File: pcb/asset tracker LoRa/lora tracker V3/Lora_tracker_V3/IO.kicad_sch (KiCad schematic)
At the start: 14 parts

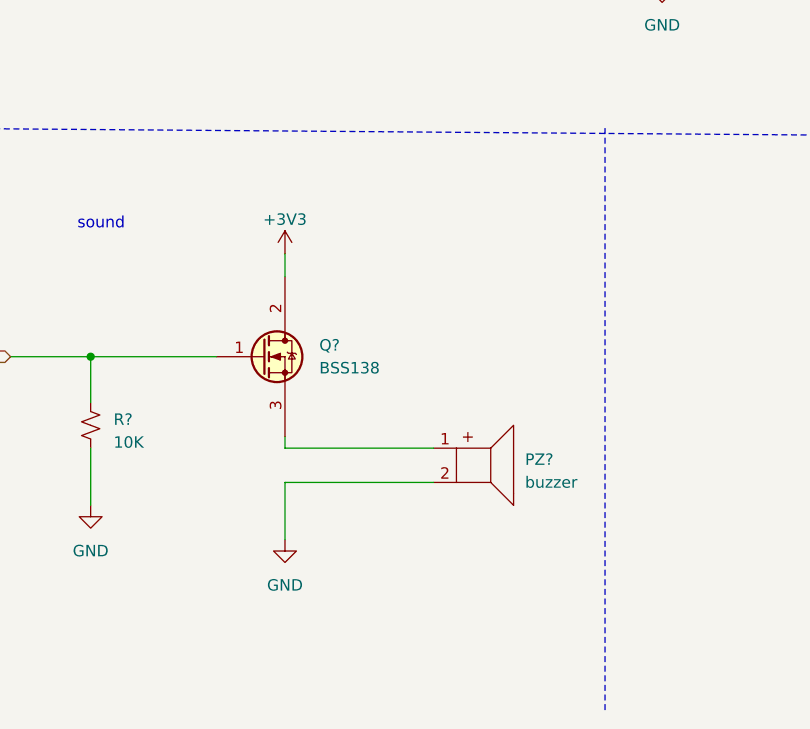
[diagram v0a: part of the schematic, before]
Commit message: sdf
fsgv
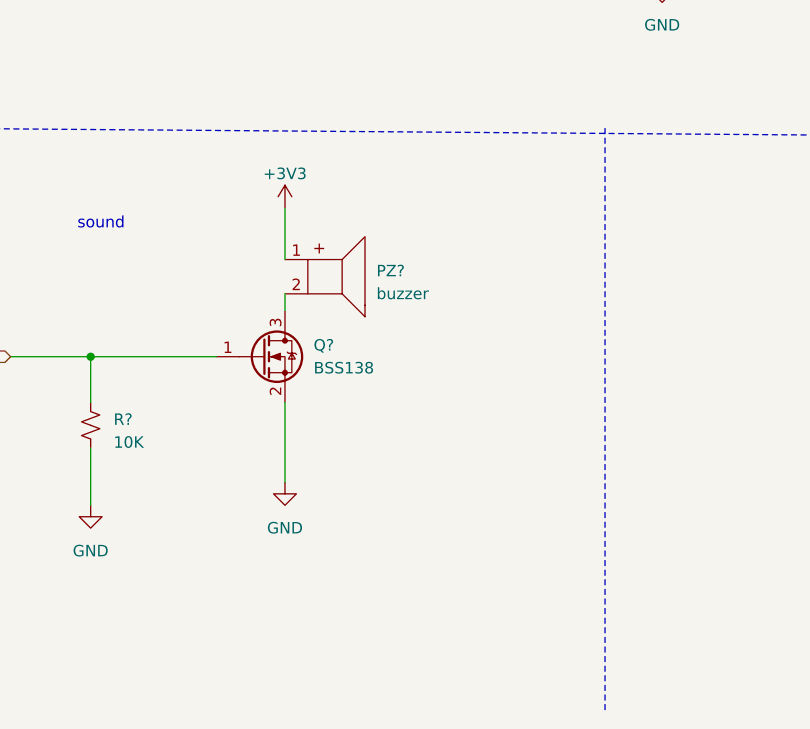
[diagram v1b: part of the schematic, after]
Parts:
- removed Q?: BSS138, halfgeleiders:sot-23,, symbol Halfgelijders:BSS138
- added Q?: BSS138, Package_TO_SOT_SMD:SOT-23, symbol Transistor_FET:BSS138
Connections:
- net +3V3: now also PZ?.1
- net BUZZER: now also Q?.1 (G)
- net GND: now also Q?.2 (S); no longer PZ?.2
- new net: PZ?.2, Q?.3 (D)
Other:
- moved on the sheet: PZ?
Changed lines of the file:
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@@
     (stroke (width 0) (type solid) (color 0 0 0 0))
   )
-  (wire (pts (xy 55.245 148.59) (xy 55.245 151.13))
-    (stroke (width 0) (type solid) (color 0 0 0 0))
-  )
-  (wire (pts (xy 55.245 168.91) (xy 55.245 170.18))
-    (stroke (width 0) (type solid) (color 0 0 0 0))
-  )
-  (wire (pts (xy 55.245 170.18) (xy 71.755 170.18))
-    (stroke (width 0) (type solid) (color 0 0 0 0))
-  )
-  (wire (pts (xy 55.245 173.99) (xy 55.245 180.34))
+  (wire (pts (xy 55.245 143.51) (xy 55.245 149.225))
+    (stroke (width 0) (type solid) (color 0 0 0 0))
+  )
+  (wire (pts (xy 55.245 153.035) (xy 55.245 154.94))
+    (stroke (width 0) (type solid) (color 0 0 0 0))
+  )
+  (wire (pts (xy 55.245 173.99) (xy 55.245 165.1))
     (stroke (width 0) (type solid) (color 0 0 0 0))
   )
@@
   )
   (wire (pts (xy 71.755 80.01) (xy 78.105 80.01))
-    (stroke (width 0) (type solid) (color 0 0 0 0))
-  )
-  (wire (pts (xy 71.755 173.99) (xy 55.245 173.99))
     (stroke (width 0) (type solid) (color 0 0 0 0))
   )
@@
     (effects (font (size 1.27 1.27)) (justify right))
   )
-  (symbol (lib_id "power:+3V3") (at 55.245 148.59 0) (unit 1)
-    (in_bom yes) (on_board yes)
-    (property "Reference" "#PWR?" (id 0) (at 55.245 152.4 0)
-      (effects (font (size 1.27 1.27)) hide)
-    )
-    (property "Value" "+3V3" (id 1) (at 55.245 144.78 0))
-    (property "Footprint" "" (id 2) (at 55.245 148.59 0)
-      (effects (font (size 1.27 1.27)) hide)
-    )
-    (property "Datasheet" "" (id 3) (at 55.245 148.59 0)
+  (symbol (lib_id "power:+3V3") (at 55.245 143.51 0) (unit 1)
+    (in_bom yes) (on_board yes)
+    (property "Reference" "#PWR?" (id 0) (at 55.245 147.32 0)
+      (effects (font (size 1.27 1.27)) hide)
+    )
+    (property "Value" "+3V3" (id 1) (at 55.245 139.7 0))
+    (property "Footprint" "" (id 2) (at 55.245 143.51 0)
+      (effects (font (size 1.27 1.27)) hide)
+    )
+    (property "Datasheet" "" (id 3) (at 55.245 143.51 0)
       (effects (font (size 1.27 1.27)) hide)
     )
@@
     (pin "1")
   )
-  (symbol (lib_id "power:GND") (at 55.245 180.34 0) (unit 1)
-    (in_bom yes) (on_board yes)
-    (property "Reference" "#PWR?" (id 0) (at 55.245 186.69 0)
-      (effects (font (size 1.27 1.27)) hide)
-    )
-    (property "Value" "GND" (id 1) (at 55.245 185.42 0))
-    (property "Footprint" "" (id 2) (at 55.245 180.34 0)
-      (effects (font (size 1.27 1.27)) hide)
-    )
-    (property "Datasheet" "" (id 3) (at 55.245 180.34 0)
+  (symbol (lib_id "power:GND") (at 55.245 173.99 0) (unit 1)
+    (in_bom yes) (on_board yes)
+    (property "Reference" "#PWR?" (id 0) (at 55.245 180.34 0)
+      (effects (font (size 1.27 1.27)) hide)
+    )
+    (property "Value" "GND" (id 1) (at 55.245 179.07 0))
+    (property "Footprint" "" (id 2) (at 55.245 173.99 0)
+      (effects (font (size 1.27 1.27)) hide)
+    )
+    (property "Datasheet" "" (id 3) (at 55.245 173.99 0)
       (effects (font (size 1.27 1.27)) hide)
     )
@@
     (pin "2")
   )
-  (symbol (lib_id "vanalles:buzzer") (at 74.295 170.18 0) (unit 1)
-    (in_bom yes) (on_board yes) (fields_autoplaced)
-    (property "Reference" "PZ?" (id 0) (at 81.915 171.4499 0)
-      (effects (font (size 1.27 1.27)) (justify left))
-    )
-    (property "Value" "buzzer" (id 1) (at 81.915 173.9899 0)
-      (effects (font (size 1.27 1.27)) (justify left))
-    )
-    (property "Footprint" "vanalles:PROSIGNAL_ABI-017-RC" (id 2) (at 74.295 170.18 0)
-      (effects (font (size 1.27 1.27)) hide)
-    )
-    (property "Datasheet" "" (id 3) (at 74.295 170.18 0)
-      (effects (font (size 1.27 1.27)) hide)
-    )
-    (pin "1")
-    (pin "2")
-  )
-  (symbol (lib_id "Halfgelijders:BSS138") (at 53.975 160.02 0) (unit 1)
-    (in_bom yes) (on_board yes) (fields_autoplaced)
-    (property "Reference" "Q?" (id 0) (at 59.055 158.7499 0)
-      (effects (font (size 1.27 1.27)) (justify left))
-    )
-    (property "Value" "BSS138" (id 1) (at 59.055 161.2899 0)
-      (effects (font (size 1.27 1.27)) (justify left))
-    )
-    (property "Footprint" "halfgeleiders:sot-23," (id 2) (at 53.975 160.02 0)
-      (effects (font (size 1.27 1.27)) hide)
-    )
-    (property "Datasheet" "" (id 3) (at 53.975 160.02 0)
-      (effects (font (size 1.27 1.27)) hide)
-    )
-    (pin "1")
+  (symbol (lib_id "vanalles:buzzer") (at 57.785 149.225 0) (unit 1)
+    (in_bom yes) (on_board yes) (fields_autoplaced)
+    (property "Reference" "PZ?" (id 0) (at 65.405 150.4949 0)
+      (effects (font (size 1.27 1.27)) (justify left))
+    )
+    (property "Value" "buzzer" (id 1) (at 65.405 153.0349 0)
+      (effects (font (size 1.27 1.27)) (justify left))
+    )
+    (property "Footprint" "vanalles:PROSIGNAL_ABI-017-RC" (id 2) (at 57.785 149.225 0)
+      (effects (font (size 1.27 1.27)) hide)
+    )
+    (property "Datasheet" "" (id 3) (at 57.785 149.225 0)
+      (effects (font (size 1.27 1.27)) hide)
+    )
+    (pin "1")
+    (pin "2")
+  )
+  (symbol (lib_id "Transistor_FET:BSS138") (at 52.705 160.02 0) (unit 1)
+    (in_bom yes) (on_board yes) (fields_autoplaced)
+    (property "Reference" "Q?" (id 0) (at 58.42 158.7499 0)
+      (effects (font (size 1.27 1.27)) (justify left))
+    )
+    (property "Value" "BSS138" (id 1) (at 58.42 161.2899 0)
+      (effects (font (size 1.27 1.27)) (justify left))
+    )
+    (property "Footprint" "Package_TO_SOT_SMD:SOT-23" (id 2) (at 57.785 161.925 0)
+      (effects (font (size 1.27 1.27) italic) (justify left) hide)
+    )
+    (property "Datasheet" "https://www.onsemi.com/pub/Collateral/BSS138-D.PDF" (id 3) (at 52.705 160.02 0)
+      (effects (font (size 1.27 1.27)) (justify left) hide)
+    )
+    (pin "1")
